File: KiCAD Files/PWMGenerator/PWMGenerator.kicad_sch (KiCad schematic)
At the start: 24 parts, among them J1 12V DC, U1 TL074

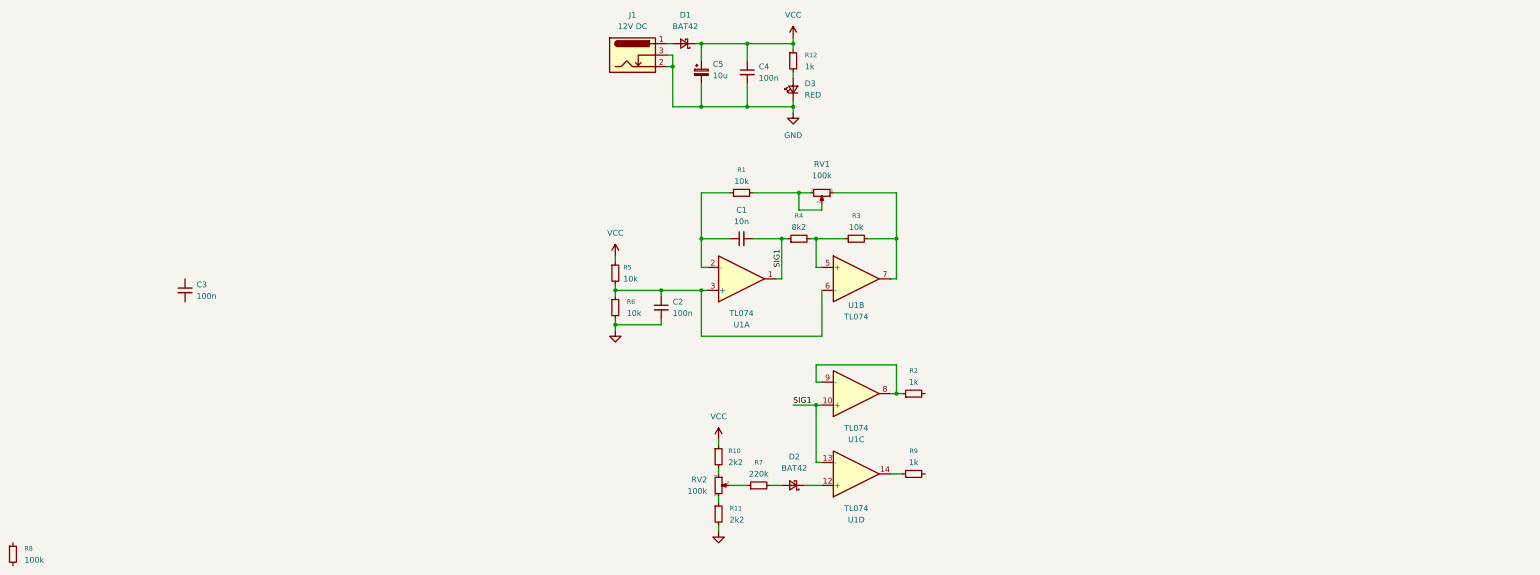
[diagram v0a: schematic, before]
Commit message: Updated Schematic
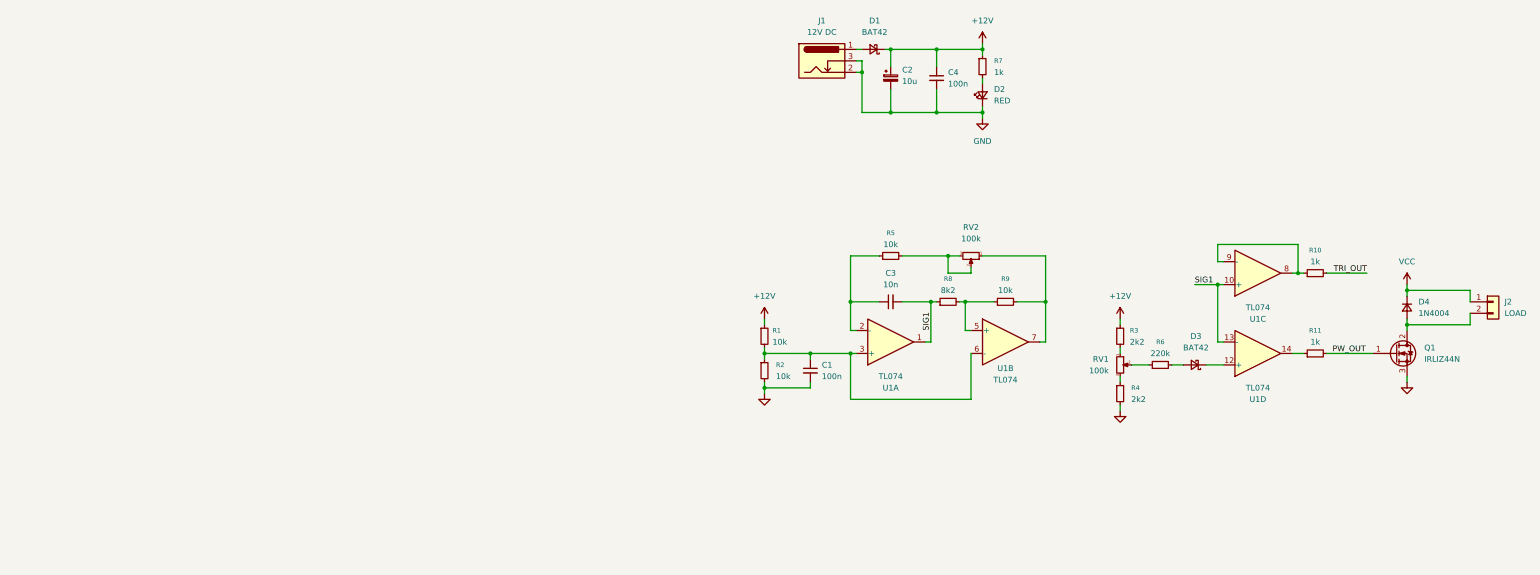
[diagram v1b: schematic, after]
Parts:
- removed C3: 100n, symbol Device:C_Small
- removed R8: 100k, symbol Device:R_Small
- added D4: 1N4004, symbol Device:D_Small
- added J2: LOAD, symbol Connector_Generic:Conn_01x02
- added Q1: IRLIZ44N, Package_TO_SOT_THT:TO-220F-3_Vertical, symbol Transistor_FET:IRLIZ44N
- renumbered C2 to C1, C5 to C2, C1 to C3, D3 to D2, D2 to D3, R5 to R1, R2 to R10, R9 to R11, R6 to R2, R10 to R3, R11 to R4, R1 to R5, R7 to R6, R12 to R7, R4 to R8, R3 to R9, RV2 to RV1, RV1 to RV2
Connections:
- net GND: now also Q1.3 (S)
- net VCC: now also D4.1 (K), J2.1 (Pin_1); no longer C2.1, C4.1, D1.1 (K), R1.1, R3.1, R7.1
- net PW_OUT: now reaches R11.2
- net PW_OUT: now also Q1.1 (G)
- net TRI_OUT: now reaches R10.2
- new net: D4.2 (A), J2.2 (Pin_2), Q1.2 (D)
- new net +12V: C2.1, C4.1, D1.1 (K), R1.1, R3.1, R7.1
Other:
- moved on the sheet: C1, C2, C3, C4, D1, D2, D3, J1, R1, R10, R11, R2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
